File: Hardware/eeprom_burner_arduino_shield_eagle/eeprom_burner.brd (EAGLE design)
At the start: 45.2 x 50 mm, 7 parts, among them IC2 74LS595N, IC3 74LS595N

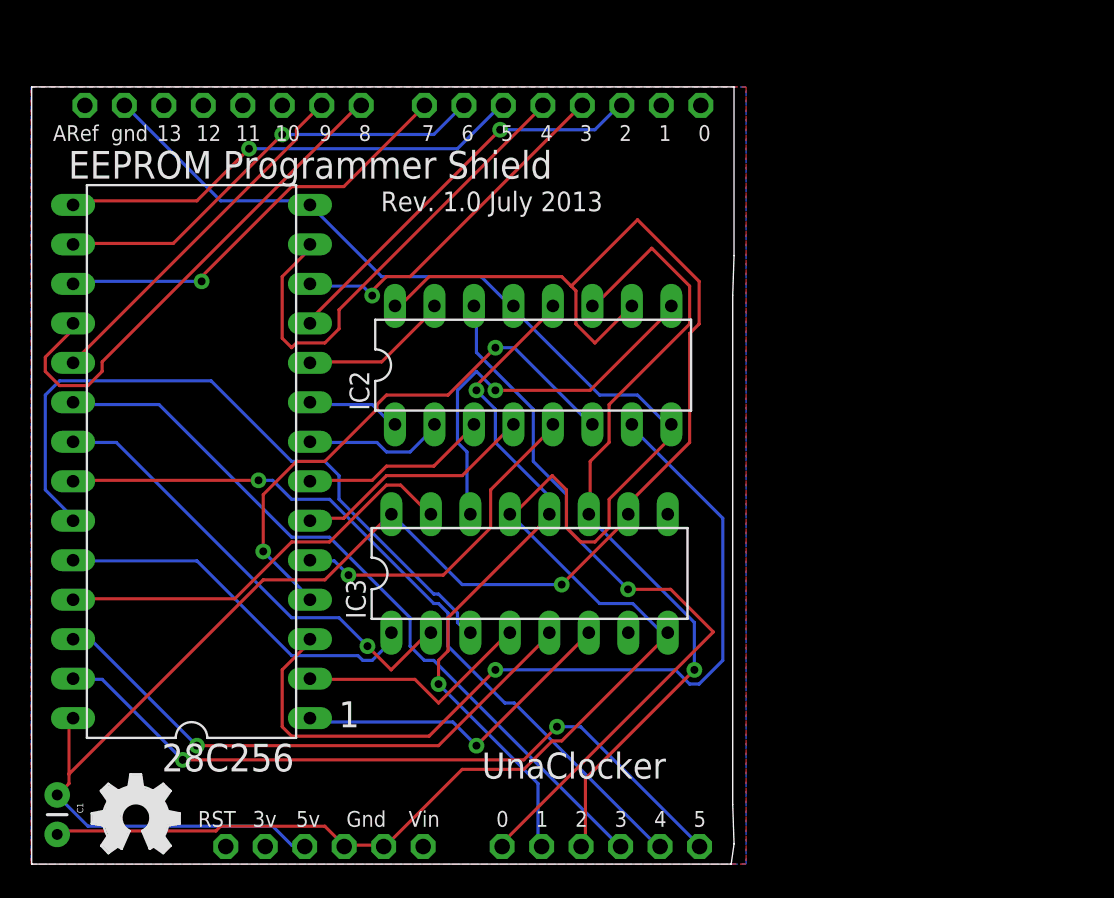
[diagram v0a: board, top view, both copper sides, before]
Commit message: updated board layout
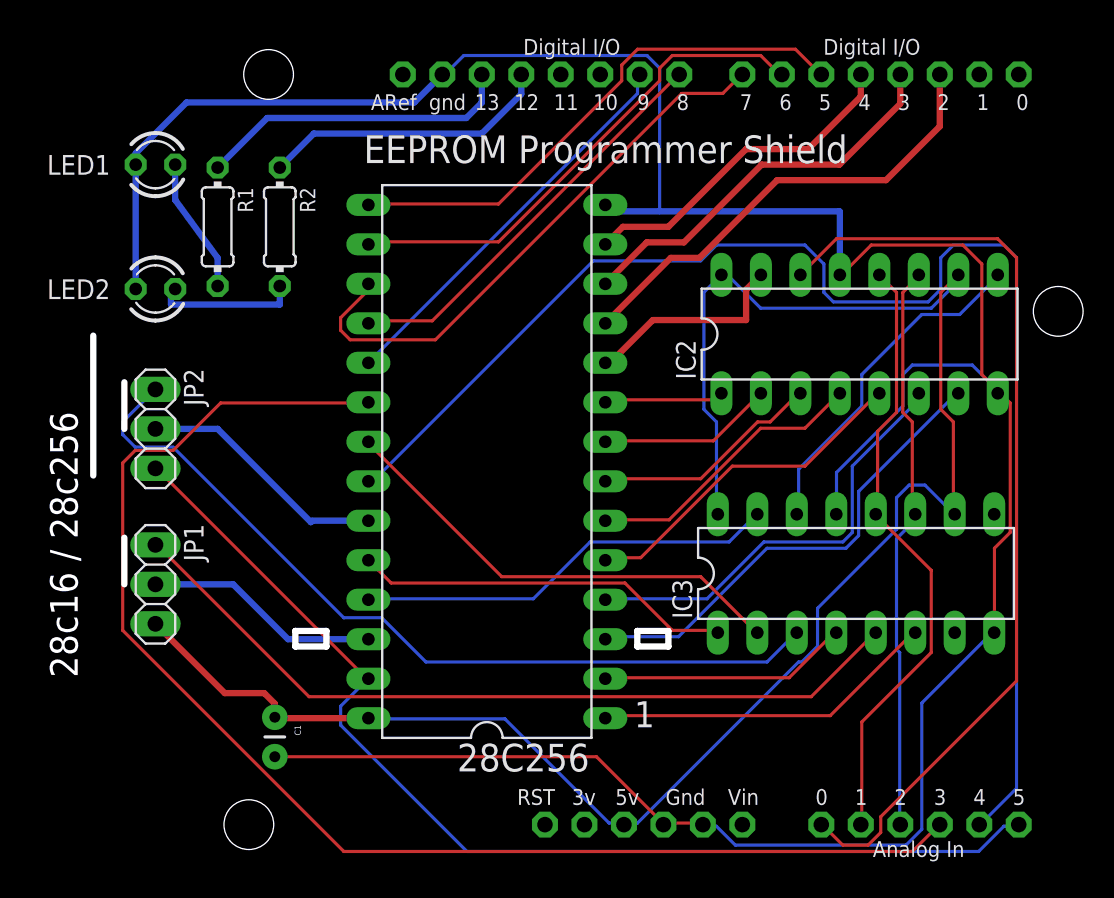
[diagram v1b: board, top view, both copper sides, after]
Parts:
- removed U$2, U$3: (no value), ohw-logo:OSHW_FILLX200_NOTEXT
- added JP1: 256 / 16 switch 1, pinhead:1X03
- added JP2: 256 / 16 switch 2, pinhead:1X03
- added LED1, LED2: (no value), led:LED3MM
- added R1, R2: 470, resistor:0204/7
- U$1: value ARDUINOUNO -> ARDUINO-NODIM; device adafruit:ARDUINO -> adafruit:ARDUINO-NODIM
- moved IC2 21.1 mm to (53.3, 34.1)
- moved IC3 21.0 mm to (53.1, 18.7)
- moved 28C256 19.0 mm to (29.3, 25.9)
- moved C1 14.9 mm to (15.7, 9.45)
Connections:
- new net A11: IC3.3, JP2.1
- new net A13: IC3.5, JP1.1
- new net N$28: LED2.A, R2.2
- new net PIN23: 28C256.23, JP2.2
- new net PIN26: 28C256.26, JP1.2
- new net WE: 28C256.27, JP2.3, U$1.A5
- net GND: now also LED1.K, LED2.K
- net N$1: now also R2.1, U$1.D12; no longer 28C256.27, U$1.A5
- net N$24: now also R1.1, U$1.D13; no longer 28C256.23, IC3.3
- net N$26: now also LED1.A, R1.2; no longer 28C256.26, IC3.5
- net VCC: now also JP1.3
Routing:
- net WE: track 0.00 -> 70.7 mm
- net GND: track 122.2 -> 187.1 mm
- net A11: track 0.00 -> 54.0 mm
- net A13: track 0.00 -> 52.1 mm
- net N$2: track 48.8 -> 91.2 mm, vias 1 -> 0
- net N$3: track 48.2 -> 87.3 mm
- net N$26: track 36.6 -> 8.70 mm, vias 1 -> 0
- net N$1: track 46.6 -> 18.8 mm, vias 2 -> 0
- net N$19: track 55.4 -> 31.0 mm, vias 1 -> 0
- net N$24: track 44.5 -> 20.5 mm
- net CLOCK: track 53.4 -> 36.8 mm, vias 1 -> 0
- net PIN23: track 0.00 -> 16.2 mm
- net PIN26: track 0.00 -> 15.2 mm
- net DS: track 48.5 -> 60.7 mm, vias 1 -> 0
- net N$28: track 0.00 -> 9.46 mm
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- removed copper zone on layer 1, net GND
- removed copper zone on layer 16, net GND
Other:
- board size 45.2 x 50 mm -> 37 x 20 mm
- board text added: "28c16 / 28c256"
- board text removed: "Rev. 1.0 July 2013"
- board text removed: "UnaClocker"
